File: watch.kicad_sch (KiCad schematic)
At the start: 1 part, among them U4 MPU-6050

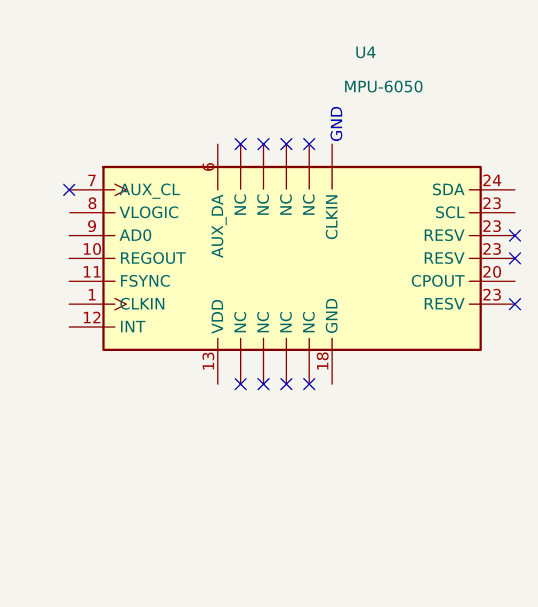
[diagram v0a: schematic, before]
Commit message: Add files via upload
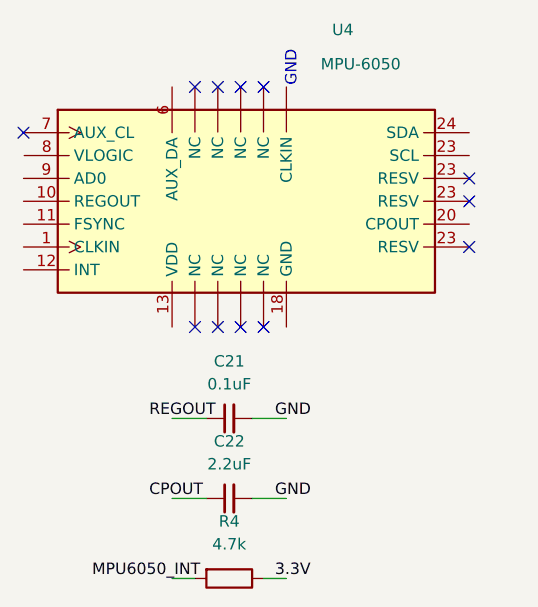
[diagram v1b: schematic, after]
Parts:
- added C21: 0.1uF_0603_16V, 4ms_Capacitor:C_0603, symbol PCM_4ms_Capacitor:0.1uF_0603_16V
- added C22: 2.2uF_0603_25V, 4ms_Capacitor:C_0603, symbol PCM_4ms_Capacitor:2.2uF_0603_25V
- added R4: 4.7k_0603, 4ms_Resistor:R_0603, symbol PCM_4ms_Resistor:4.7k_0603
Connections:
- new net 3.3V: R4.1
- new net GND: C21.2, C22.2
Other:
- moved on the sheet: U4
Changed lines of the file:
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@@
 (kicad_sch (version 20230121) (generator eeschema)
   (paper "A4")
-  (no_connect (at 72.39 38.1))
-  (no_connect (at 41.91 54.61))
-  (no_connect (at 46.99 27.94))
-  (no_connect (at 44.45 54.61))
-  (no_connect (at 49.53 27.94))
-  (no_connect (at 22.86 33.02))
-  (no_connect (at 49.53 54.61))
-  (no_connect (at 72.39 40.64))
-  (no_connect (at 72.39 45.72))
-  (no_connect (at 46.99 54.61))
-  (no_connect (at 44.45 27.94))
-  (no_connect (at 41.91 27.94))
-  (text "GND\n" (at 53.34 27.94 90)
-    (effects (font (size 1.27 1.27)) (justify left bottom))
-  )
-  (symbol (lib_id "Sensor_Motion:MPU-6050") (at 46.99 40.64 0) (unit 1)
-    (in_bom yes) (on_board yes) (dnp no) (fields_autoplaced)
-    (property "Reference" "U4" (at 54.61 17.78 0)
+  (no_connect (at 67.31 31.75))
+  (no_connect (at 36.83 48.26))
+  (no_connect (at 41.91 21.59))
+  (no_connect (at 39.37 48.26))
+  (no_connect (at 44.45 21.59))
+  (no_connect (at 17.78 26.67))
+  (no_connect (at 44.45 48.26))
+  (no_connect (at 67.31 34.29))
+  (no_connect (at 67.31 39.37))
+  (no_connect (at 41.91 48.26))
+  (no_connect (at 39.37 21.59))
+  (no_connect (at 36.83 21.59))
+  (wire (pts (xy 44.45 76.2) (xy 46.99 76.2))
+    (stroke (width 0) (type default))
+  )
+  (wire (pts (xy 43.18 67.31) (xy 46.99 67.31))
+    (stroke (width 0) (type default))
+  )
+  (wire (pts (xy 43.18 58.42) (xy 46.99 58.42))
+    (stroke (width 0) (type default))
+  )
+  (wire (pts (xy 34.29 67.31) (xy 38.1 67.31))
+    (stroke (width 0) (type default))
+  )
+  (wire (pts (xy 34.29 58.42) (xy 38.1 58.42))
+    (stroke (width 0) (type default))
+  )
+  (wire (pts (xy 34.29 76.2) (xy 36.83 76.2))
+    (stroke (width 0) (type default))
+  )
+  (text "GND\n" (at 48.26 21.59 90)
+    (effects (font (size 1.27 1.27)) (justify left bottom))
+  )
+  (label "3.3V" (at 45.72 76.2 0) (fields_autoplaced)
+    (effects (font (size 1.27 1.27)) (justify left bottom))
+  )
+  (label "REGOUT" (at 31.75 58.42 0) (fields_autoplaced)
+    (effects (font (size 1.27 1.27)) (justify left bottom))
+  )
+  (label "CPOUT" (at 31.75 67.31 0) (fields_autoplaced)
+    (effects (font (size 1.27 1.27)) (justify left bottom))
+  )
+  (label "MPU6050_INT" (at 25.4 76.2 0) (fields_autoplaced)
+    (effects (font (size 1.27 1.27)) (justify left bottom))
+  )
+  (label "GND" (at 45.72 58.42 0) (fields_autoplaced)
+    (effects (font (size 1.27 1.27)) (justify left bottom))
+  )
+  (label "GND" (at 45.72 67.31 0) (fields_autoplaced)
+    (effects (font (size 1.27 1.27)) (justify left bottom))
+  )
+  (symbol (lib_id "Sensor_Motion:MPU-6050") (at 41.91 34.29 0) (unit 1)
+    (in_bom yes) (on_board yes) (dnp no)
+    (property "Reference" "U4" (at 52.07 15.24 0)
       (effects (font (size 1.27 1.27)) (justify left))
     )
-    (property "Value" "MPU-6050" (at 53.34 21.59 0)
+    (property "Value" "MPU-6050" (at 50.8 19.05 0)
       (effects (font (size 1.27 1.27)) (justify left))
     )
-    (property "Footprint" "Sensor_Motion:InvenSense_QFN-24_4x4mm_P0.5mm" (at 86.36 16.51 0)
-      (effects (font (size 1.27 1.27)) hide)
-    )
-    (property "Datasheet" "https://invensense.tdk.com/wp-content/uploads/2015/02/MPU-6000-Datasheet1.pdf" (at 95.25 19.05 0)
+    (property "Footprint" "Sensor_Motion:InvenSense_QFN-24_4x4mm_P0.5mm" (at 81.28 10.16 0)
+      (effects (font (size 1.27 1.27)) hide)
+    )
+    (property "Datasheet" "https://invensense.tdk.com/wp-content/uploads/2015/02/MPU-6000-Datasheet1.pdf" (at 90.17 12.7 0)
       (effects (font (size 1.27 1.27)) hide)
     )
@@
         )
       )
+    )
+  )
+  (symbol (lib_id "PCM_4ms_Capacitor:0.1uF_0603_16V") (at 40.64 58.42 90) (unit 1)
+    (in_bom yes) (on_board yes) (dnp no) (fields_autoplaced)
+    (property "Reference" "C21" (at 40.6463 52.07 90)
+      (effects (font (size 1.27 1.27)))
+    )
+    (property "Value" "0.1uF_0603_16V" (at 36.83 58.42 0)
+      (effects (font (size 1.27 1.27)) hide)
+    )
+    (property "Footprint" "4ms_Capacitor:C_0603" (at 45.72 60.96 0)
+      (effects (font (size 1.27 1.27)) (justify left) hide)
+    )
+    (property "Datasheet" "" (at 40.64 58.42 0)
+      (effects (font (size 1.27 1.27)) hide)
+    )
+    (property "Specifications" "0.1uF, Min. 16V 10%, X7R or X5R or similar" (at 48.514 60.96 0)
+      (effects (font (size 1.27 1.27)) (justify left) hide)
+    )
+    (property "Manufacturer" "AVX Corporation" (at 50.038 60.96 0)
+      (effects (font (size 1.27 1.27)) (justify left) hide)
+    )
+    (property "Part Number" "0603YC104KAT2A" (at 51.562 60.96 0)
+      (effects (font (size 1.27 1.27)) (justify left) hide)
+    )
+    (property "Display" "0.1uF" (at 40.6463 54.61 90)
+      (effects (font (size 1.27 1.27)))
+    )
+    (property "JLCPCB ID" "C14663" (at 53.34 57.15 0)
+      (effects (font (size 1.27 1.27)) hide)
+    )
+    (pin "1")
+    (pin "2")
+    (instances
+      (project "watch"
+        (path "/d585b074-b42a-4769-9922-82a29abf42b8"
+          (reference "C21") (unit 1)
+        )
+      )
+    )
+  )
+  (symbol (lib_id "PCM_4ms_Resistor:4.7k_0603") (at 40.64 76.2 270) (unit 1)
+    (in_bom yes) (on_board yes) (dnp no)
+    (property "Reference" "R4" (at 40.64 69.85 90)
+      (effects (font (size 1.27 1.27)))
+    )
+    (property "Value" "4.7k_0603" (at 40.64 73.66 90)
+      (effects (font (size 1.27 1.27)) hide)
+    )
+    (property "Footprint" "4ms_Resistor:R_0603" (at 27.94 73.66 0)
+      (effects (font (size 1.27 1.27)) (justify left) hide)
+    )
+    (property "Datasheet" "" (at 40.64 76.2 0)
+      (effects (font (size 1.27 1.27)) hide)
+    )
+    (property "Specifications" "4k7, 1%, 1/10W, 0603" (at 32.766 73.66 0)
+      (effects (font (size 1.27 1.27)) (justify left) hide)
+    )
+    (property "Manufacturer" "Yageo" (at 31.242 73.66 0)
+      (effects (font (size 1.27 1.27)) (justify left) hide)
+    )
+    (property "Part Number" "RC0603FR-074K7L" (at 29.718 73.66 0)
+      (effects (font (size 1.27 1.27)) (justify left) hide)
+    )
+    (property "Display" "4.7k" (at 40.64 72.39 90)
+      (effects (font (size 1.27 1.27)))
+    )
+    (property "JLCPCB ID" "C23162" (at 40.64 76.2 0)
+      (effects (font (size 1.27 1.27)) hide)
+    )
+    (pin "1")
+    (pin "2")
+    (instances
+      (project "watch"
+        (path "/d585b074-b42a-4769-9922-82a29abf42b8"
+          (reference "R4") (unit 1)
+        )
+      )
+    )
+  )
+  (symbol (lib_id "PCM_4ms_Capacitor:2.2uF_0603_25V") (at 40.64 67.31 90) (unit 1)
+    (in_bom yes) (on_board yes) (dnp no) (fields_autoplaced)
+    (property "Reference" "C22" (at 40.6463 60.96 90)
+      (effects (font (size 1.27 1.27)))
+    )
+    (property "Value" "2.2uF_0603_25V" (at 36.83 67.31 0)
+      (effects (font (size 1.27 1.27)) hide)
+    )
+    (property "Footprint" "4ms_Capacitor:C_0603" (at 53.34 59.055 0)
+      (effects (font (size 1.27 1.27)) hide)
+    )
+    (property "Datasheet" "" (at 40.64 67.31 0)
+      (effects (font (size 1.27 1.27)) hide)
+    )
+    (property "Specifications" "2.2uF, Min 25V 10% X5R" (at 48.514 69.85 0)
+      (effects (font (size 1.27 1.27)) (justify left) hide)
+    )
+    (property "Manufacturer" "Murata" (at 50.038 69.85 0)
+      (effects (font (size 1.27 1.27)) (justify left) hide)
+    )
+    (property "Part Number" "GRM188R6YA225KA12D" (at 51.562 69.85 0)
+      (effects (font (size 1.27 1.27)) (justify left) hide)
+    )
+    (property "Display" "2.2uF" (at 40.6463 63.5 90)
+      (effects (font (size 1.27 1.27)))
+    )
+    (property "JLCPCB ID" "C57895" (at 40.64 67.31 0)
+      (effects (font (size 1.27 1.27)) hide)
+    )
+    (pin "1")
+    (pin "2")
+    (instances
+      (project "watch"
+        (path "/d585b074-b42a-4769-9922-82a29abf42b8"
+          (reference "C22") (unit 1)
+        )
+      )
